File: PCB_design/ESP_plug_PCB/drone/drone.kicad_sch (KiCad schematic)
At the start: 67 parts, among them J1 USB_B_Micro, J11 Conn_2, J16 Conn_2, J2 Conn_01x09, J21 Conn_2, J23 Conn_01x02_Pin, J24 Conn_01x08, J4 Conn_2, Q1 AO3400A, Q2 AO3400A, Q3 AO3400A, Q4 AO3400A, Q6 AO3401A, SW1 SW_Push, SW3 SW_Push, U1 ESP32-S3-MINI-1, U2 USBLC6-2SC6, U3 CP2102N-A02-GQFN28, U4 BC847CDW1T1G, U5 AP2112K-3.3TRG1, U6 MPU-6050

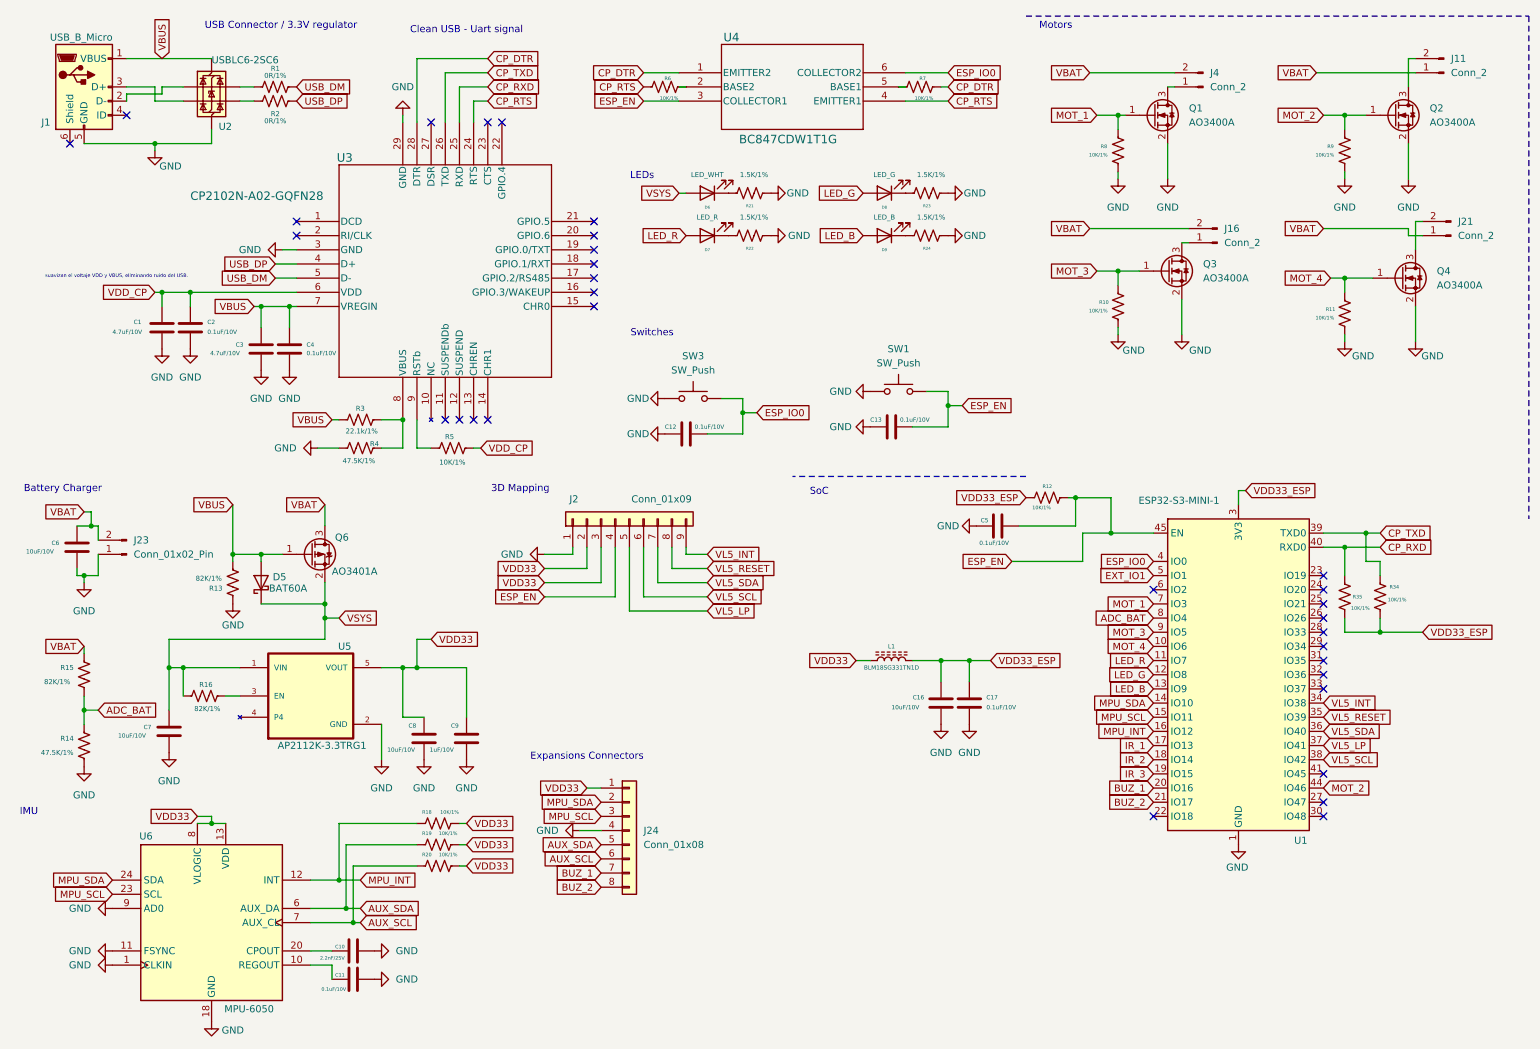
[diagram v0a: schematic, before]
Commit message: Pcb with holes
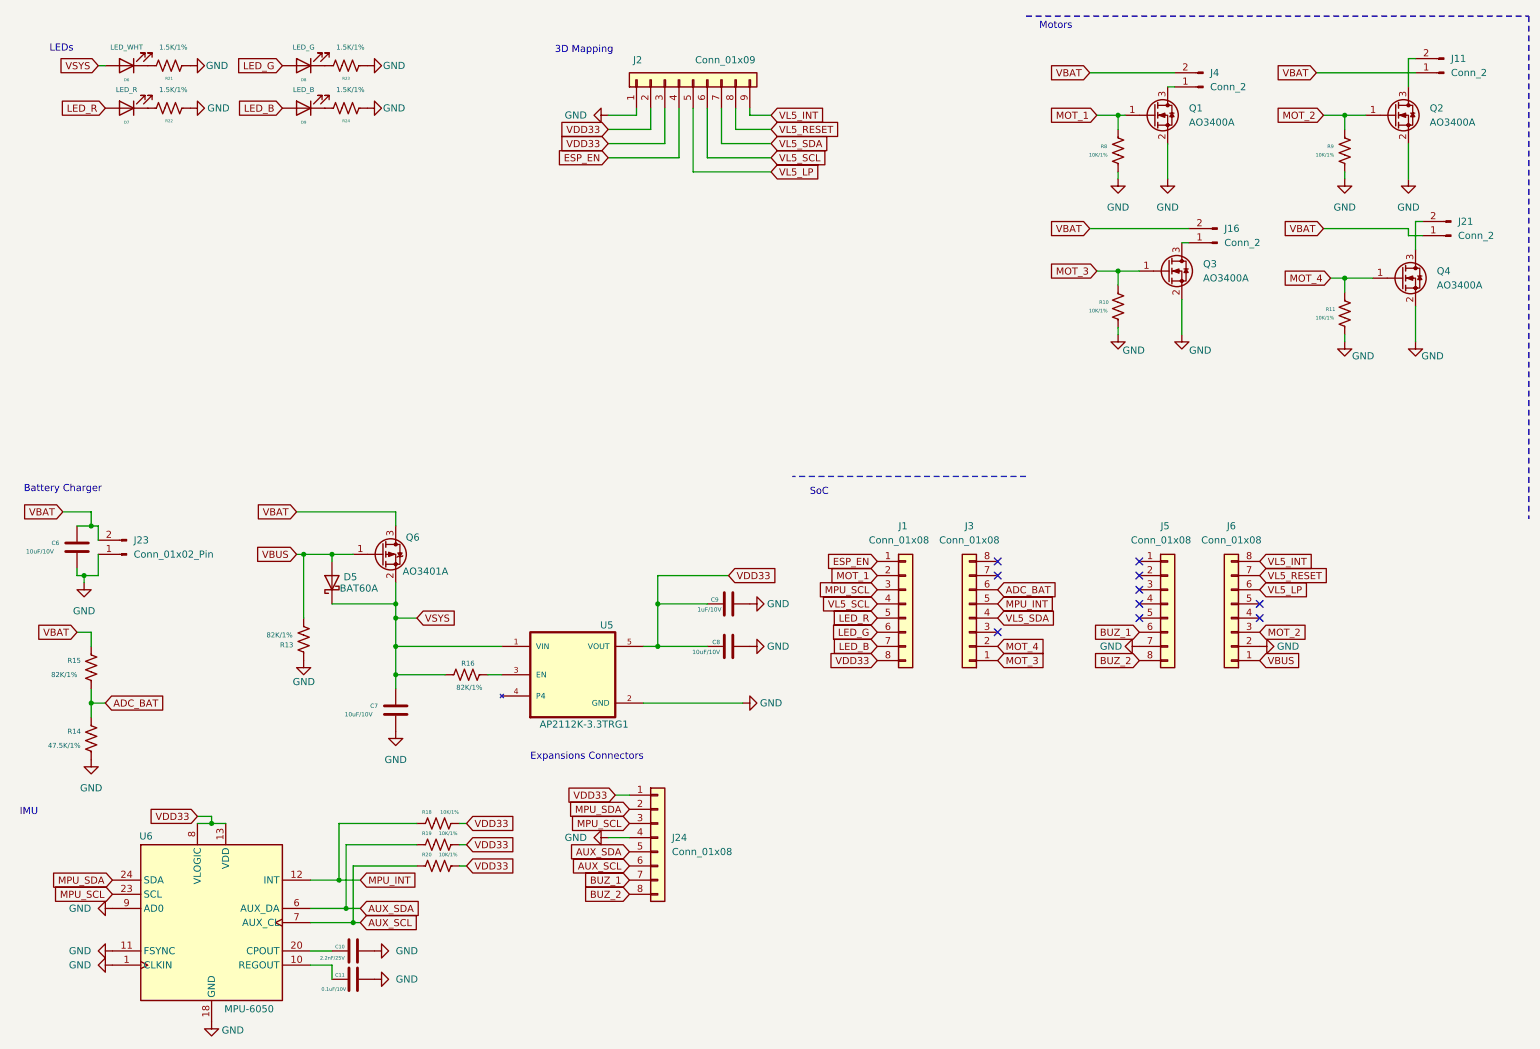
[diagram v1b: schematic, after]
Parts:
- removed C1, C3: 4.7uF/10V, Capacitor_SMD:C_0201_0603Metric, symbol Device:C
- removed C12, C13, C17, C2, C4, C5: 0.1uF/10V, Capacitor_SMD:C_0201_0603Metric, symbol Device:C
- removed C16: 10uF/10V, Capacitor_SMD:C_0201_0603Metric, symbol Device:C
- removed J1: USB_B_Micro, Connector_USB:USB_Micro-B_Amphenol_10118193-0002LF_Horizontal, symbol Connector:USB_B_Micro
- removed L1: BLM18SG331TN1D, Inductor_SMD:L_0201_0603Metric, symbol Device:L_Ferrite
- removed R1, R2: 0R/1%, Resistor_SMD:R_0201_0603Metric, symbol Device:R_US
- removed R12, R34, R35, R5, R6, R7: 10K/1%, Resistor_SMD:R_0201_0603Metric, symbol Device:R_US
- removed R3: 22.1k/1%, Resistor_SMD:R_0201_0603Metric, symbol Device:R_US
- removed R4: 47.5K/1%, Resistor_SMD:R_0201_0603Metric, symbol Device:R_US
- removed SW1: SW_Push, Button_Switch_SMD:SW_DIP_SPSTx01_Slide_6.7x4.1mm_W8.61mm_P2.54mm_LowProfile, symbol Switch:SW_Push
- removed SW3: SW_Push, Button_Switch_THT:SW_Tactile_SPST_Angled_PTS645Vx39-2LFS, symbol Switch:SW_Push
- removed U1: ESP32-S3-MINI-1, RF_Module:ESP32-S2-MINI-1, symbol MCU_Espressif:ESP32-S3-MINI-1
- removed U2: USBLC6-2SC6, Package_TO_SOT_SMD:SOT-23-6, symbol Power_Protection:USBLC6-2SC6
- removed U3: CP2102N-A02-GQFN28, usb_bridge:CP2102N-A02-GQFN28, symbol 2026-03-03_10-35-32:CP2102N-A02-GQFN28
- removed U4: BC847CDW1T1G, transistor:BC847CDW1T1G, symbol 2026-03-07_16-08-08:BC847CDW1T1G
- added J1, J3, J5, J6: Conn_01x08, Connector_PinHeader_2.54mm:PinHeader_1x08_P2.54mm_Vertical, symbol Connector_Generic:Conn_01x08
- J11, J16, J21, J4: footprint Connector_PinSocket_2.00mm:PinSocket_1x02_P2.00mm_Horizontal -> Connector_JST:JST_XH_S2B-XH-A-1_1x02_P2.50mm_Horizontal
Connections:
- net ADC_BAT: now also J3.6 (Pin_6)
- net BUZ_1: now also J5.6 (Pin_6)
- net BUZ_2: now also J5.8 (Pin_8)
- net ESP_EN: now also J1.1 (Pin_1)
- net GND: now also J5.7 (Pin_7), J6.2 (Pin_2)
- net LED_B: now also J1.7 (Pin_7)
- net LED_G: now also J1.6 (Pin_6)
- net LED_R: now also J1.5 (Pin_5)
- net MOT_1: now also J1.2 (Pin_2)
- net MOT_2: now also J6.3 (Pin_3)
- net MOT_3: now also J3.1 (Pin_1)
- net MOT_4: now also J3.2 (Pin_2)
- net MPU_INT: now also J3.5 (Pin_5)
- net MPU_SCL: now also J1.3 (Pin_3)
- net VBUS: now also J6.1 (Pin_1)
- net VDD33: now also J1.8 (Pin_8)
- net VL5_INT: now also J6.8 (Pin_8)
- net VL5_LP: now also J6.6 (Pin_6)
- net VL5_RESET: now also J6.7 (Pin_7)
- net VL5_SCL: now also J1.4 (Pin_4)
- net VL5_SDA: now also J3.4 (Pin_4)
- no-connect marks 32 -> 10
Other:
- note removed: "Clean USB - Uart signal"
- note removed: "Switches"
- note removed: "USB Connector / 3.3V regulator"
- note removed: "suavizan el voltaje VDD y VBUS, eliminando ruido del USB."
- moved on the sheet: C7, C8, C9, D5, D6, D7, D8, D9, J2, J24, Q6, R13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

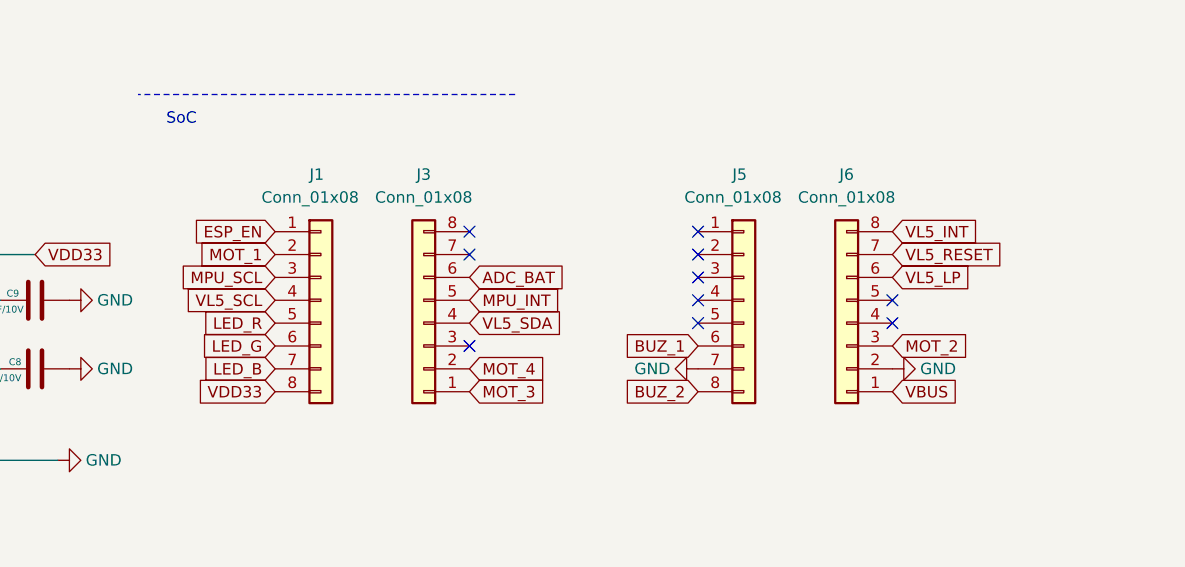
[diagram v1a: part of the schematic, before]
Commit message: fix
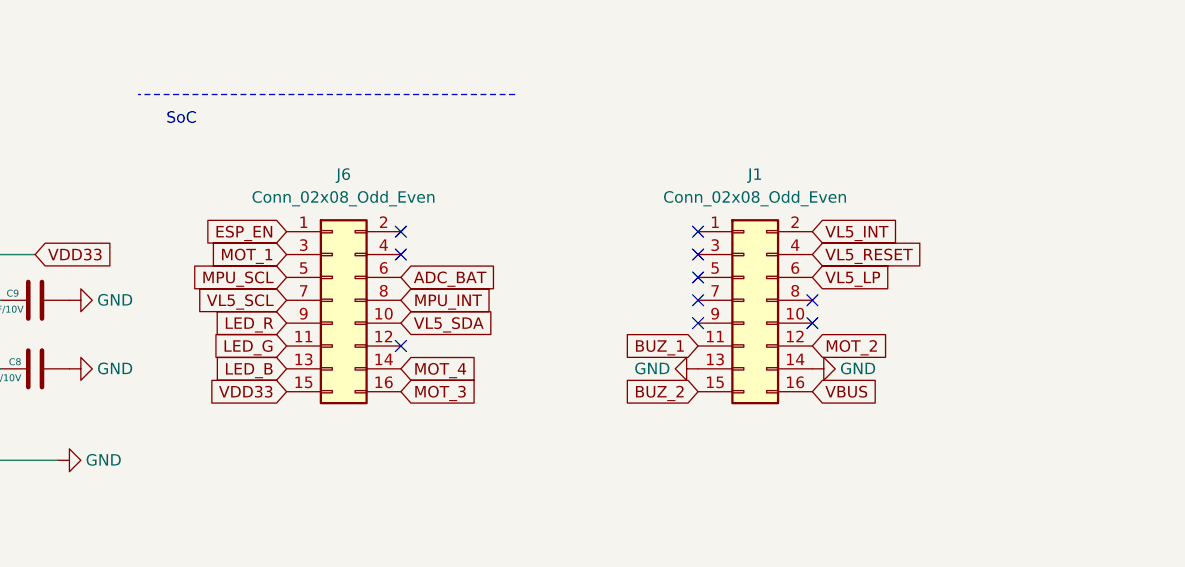
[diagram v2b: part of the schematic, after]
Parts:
- removed J1, J3, J5, J6: Conn_01x08, Connector_PinHeader_2.54mm:PinHeader_1x08_P2.54mm_Vertical, symbol Connector_Generic:Conn_01x08
- added J1, J6: Conn_02x08_Odd_Even, Connector_PinHeader_2.54mm:PinHeader_2x08_P2.54mm_Vertical, symbol Connector_Generic:Conn_02x08_Odd_Even
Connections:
- net ADC_BAT: now also J6.6 (Pin_6)
- net BUZ_1: now also J1.11 (Pin_11)
- net BUZ_2: now also J1.15 (Pin_15)
- net ESP_EN: now also J6.1 (Pin_1)
- net GND: now also J1.13 (Pin_13), J1.14 (Pin_14)
- net LED_B: now also J6.13 (Pin_13)
- net LED_G: now also J6.11 (Pin_11)
- net LED_R: now also J6.9 (Pin_9)
- net MOT_1: now also J6.3 (Pin_3)
- net MOT_2: now also J1.12 (Pin_12)
- net MOT_3: now also J6.16 (Pin_16)
- net MOT_4: now also J6.14 (Pin_14)
- net MPU_INT: now also J6.8 (Pin_8)
- net MPU_SCL: now also J6.5 (Pin_5)
- net VBUS: now also J1.16 (Pin_16)
- net VDD33: now also J6.15 (Pin_15)
- net VL5_INT: now also J1.2 (Pin_2)
- net VL5_LP: now also J1.6 (Pin_6)
- net VL5_RESET: now also J1.4 (Pin_4)
- net VL5_SCL: now also J6.7 (Pin_7)
- net VL5_SDA: now also J6.10 (Pin_10)

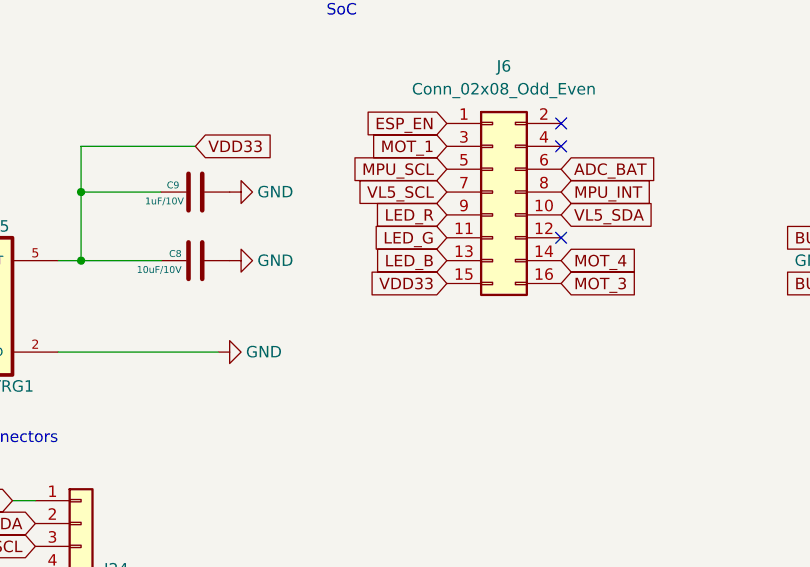
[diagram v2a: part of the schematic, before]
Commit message: Fix 3.3v
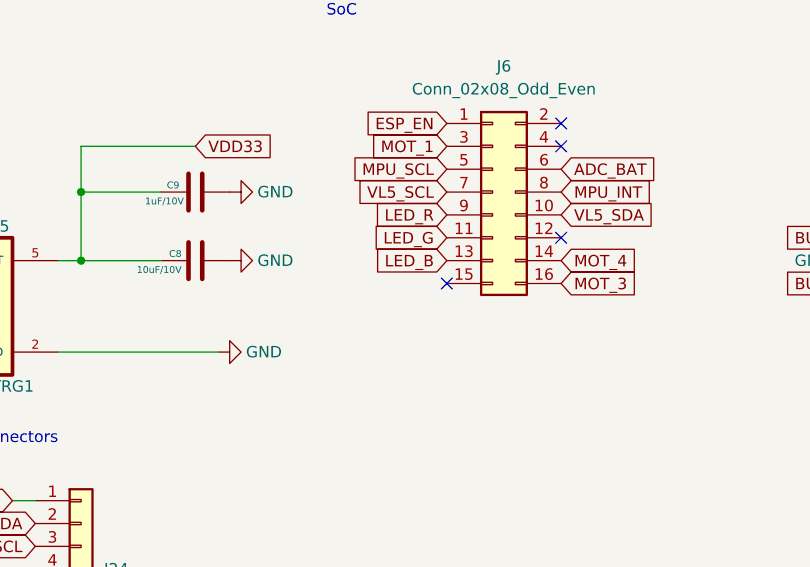
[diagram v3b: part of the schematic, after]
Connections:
- net VDD33: no longer J6.15 (Pin_15)
- no-connect marks 10 -> 11
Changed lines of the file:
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@@
 		(at 214.63 113.03)
+	)
+	(no_connect
+		(at 168.91 128.27)
 	)
 	(wire
@@
 				(hide yes)
 			)
-		)
-	)
-	(global_label "VDD33"
-		(shape input)
-		(at 168.91 128.27 180)
-		(fields_autoplaced yes)
-		(effects
-			(font
-				(size 1.27 1.27)
-			)
-			(justify right)
-		)
-		(property "Intersheetrefs" "${INTERSHEET_REFS}"
-			(at 159.8772 128.27 0)
-			(effects
-				(font
-					(size 1.27 1.27)
-				)
-				(justify right)
-				(hide yes)
-			)
